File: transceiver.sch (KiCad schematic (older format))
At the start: 18 parts, among them U3 CC1200, Y1 Crystal_GND23

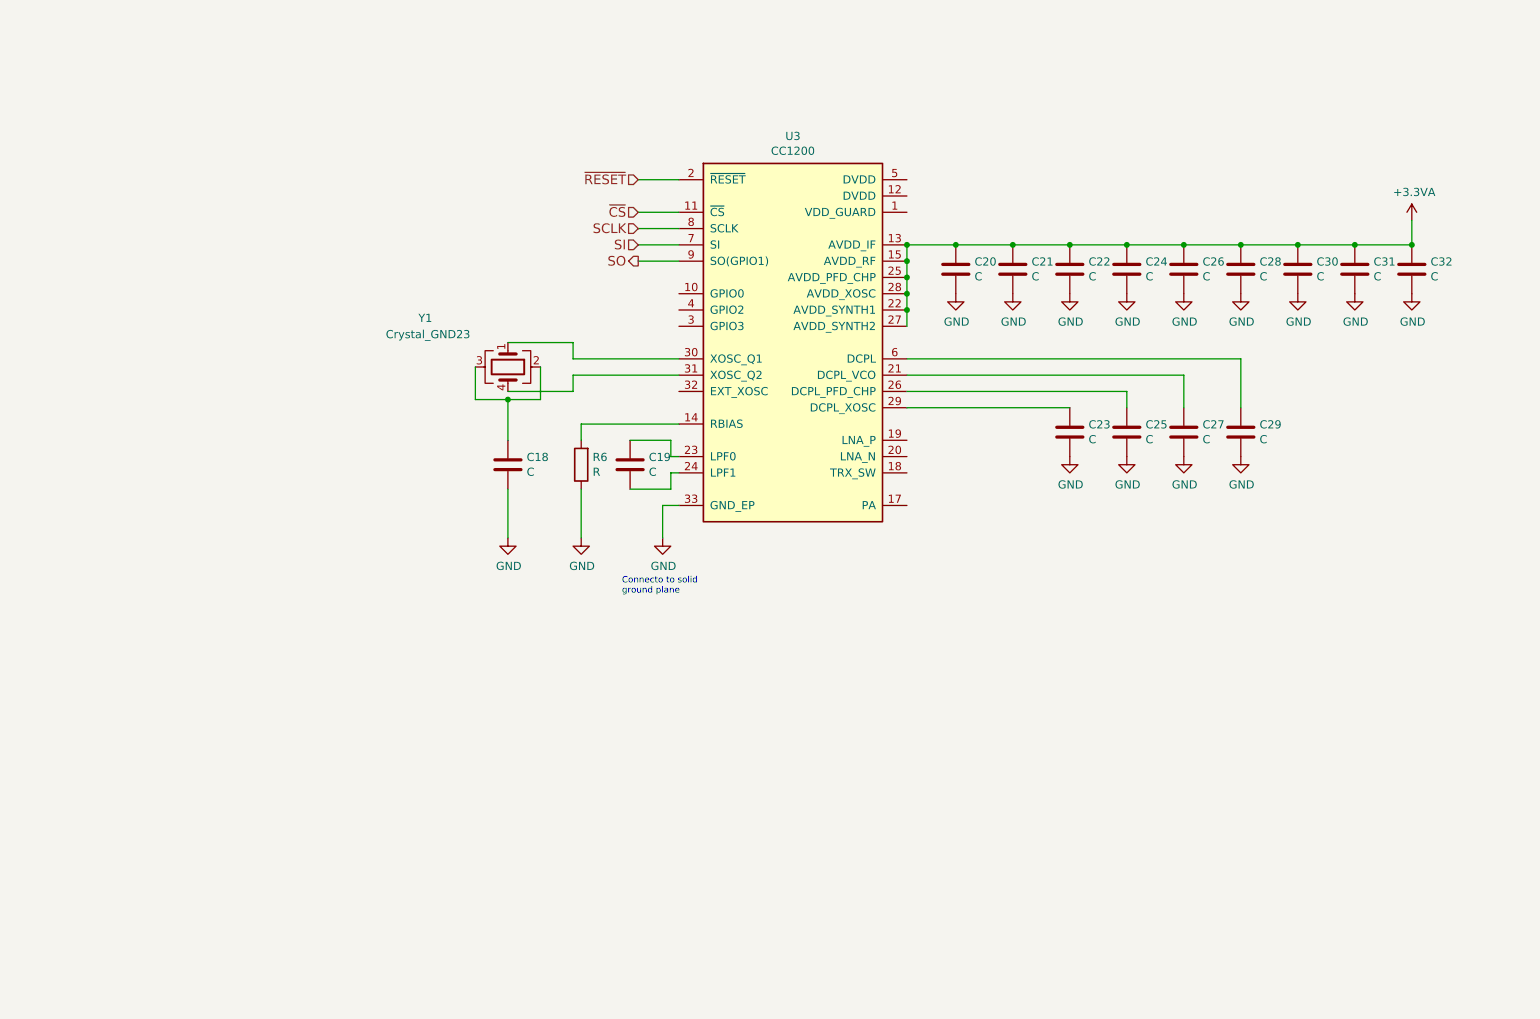
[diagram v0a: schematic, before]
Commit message: More work on tranciever and PA
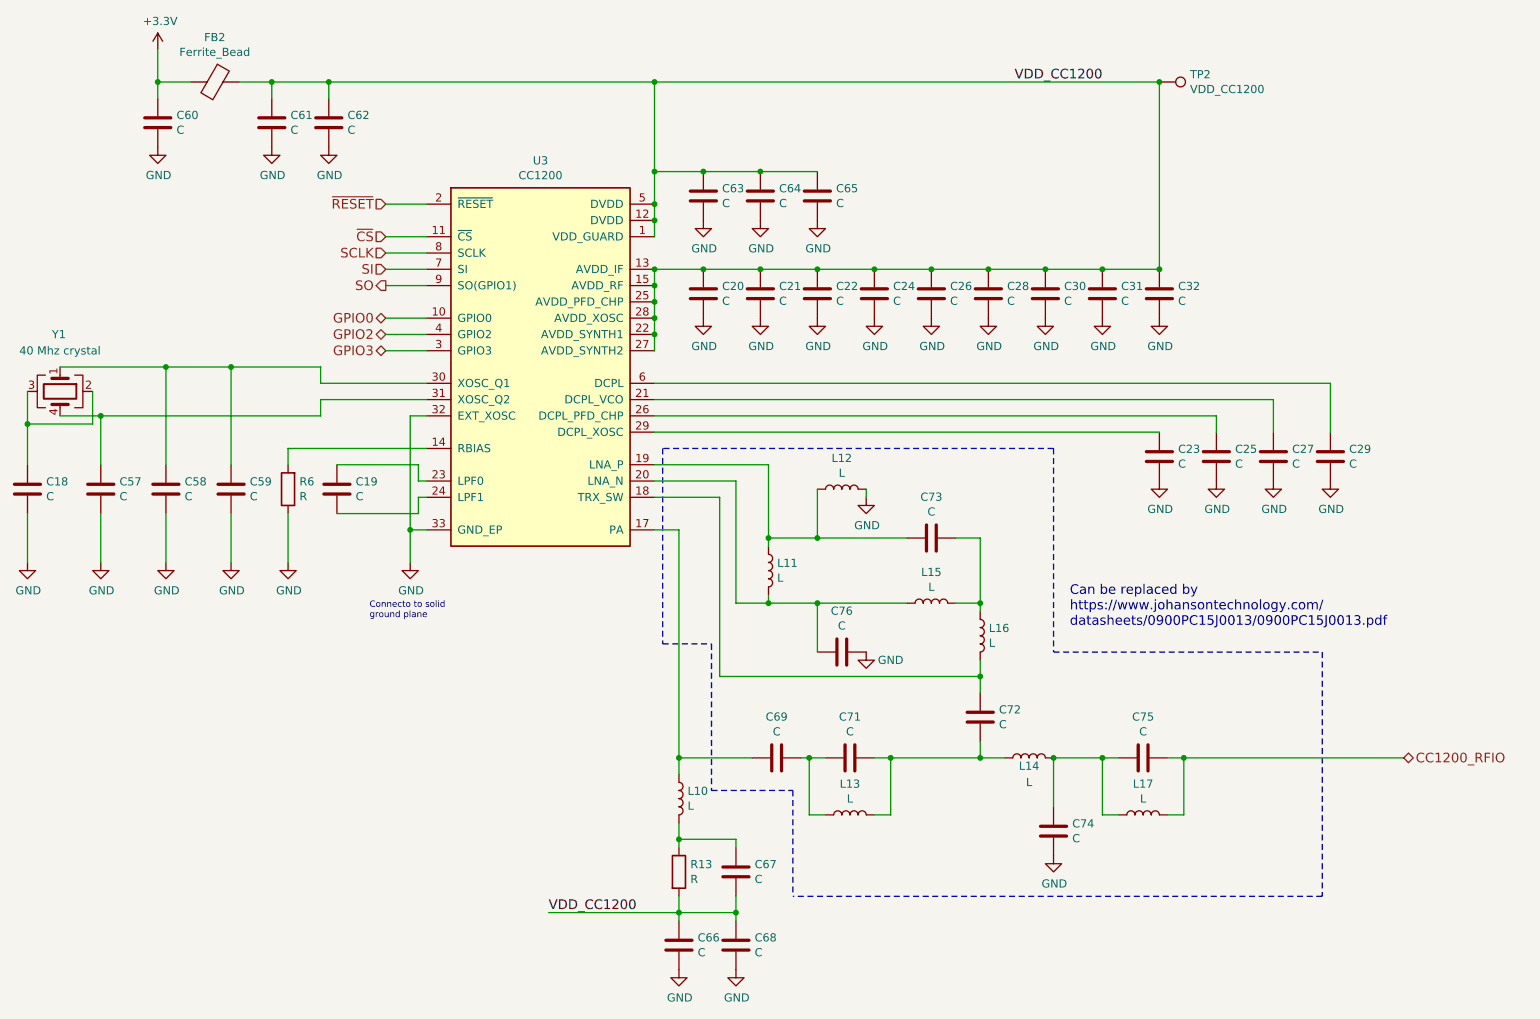
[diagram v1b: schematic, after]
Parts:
- added C57, C58, C59, C60, C61, C62, C63, C64, C65, C66, C67, C68, C69, C71, C72, C73, C74, C75, C76: C, symbol Device:C
- added FB2: Ferrite_Bead, symbol Device:Ferrite_Bead
- added L10, L11, L12, L13, L14, L15, L16, L17: L, symbol Device:L
- added R13: R, symbol Device:R
- added TP2: VDD_CC1200, symbol Connector:TestPoint
- Y1: value Crystal_GND23 -> 40 Mhz crystal
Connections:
- net +3.3VA is gone; now on net VDD_CC1200: C20.1, C21.1, C22.1, C24.1, C26.1, C28.1, C30.1, C31.1, C32.1, U3.13 (AVDD_IF), U3.15 (AVDD_RF), U3.22 (AVDD_SYNTH1), U3.25 (AVDD_PFD_CHP), U3.27 (AVDD_SYNTH2), U3.28 (AVDD_XOSC)
- net GND: now also U3.32 (EXT_XOSC), C57.2, C58.2, C59.2, C60.2, C61.2, C62.2, C63.2, C64.2, C65.2, C66.2, C68.2, C74.2, C76.1, L12.2
- net VDD_CC1200: now reaches U3.1 (VDD_GUARD)
- net VDD_CC1200: now also U3.12 (DVDD), U3.5 (DVDD), C61.1, C62.1, C63.1, C64.1, C65.1, C66.1, C67.2, C68.1, FB2.1, R13.2, TP2.1
- net GPIO0: now reaches U3.10 (GPIO0)
- net at U3.17 (PA): now also C69.2, L10.1
- net at U3.18 (TRX_SW): now also C72.1, L16.2
- net at U3.19 (LNA_P): now also C73.2, L11.1, L12.1
- net at U3.20 (LNA_N): now also C76.2, L11.2, L15.1
- net GPIO3: now reaches U3.3 (GPIO3)
- net at U3.30 (XOSC_Q1), Y1.1: now also C58.1, C59.1
- net at U3.31 (XOSC_Q2), Y1.4: now also C57.1
- net GPIO2: now reaches U3.4 (GPIO2)
- new net: C67.1, L10.2, R13.1
- new net: C69.1, C71.2, L13.1
- new net: C71.1, C72.2, L13.2, L14.1
- new net: C74.1, C75.2, L14.2, L17.1
- new net: C73.1, L15.2, L16.1
- new net +3V3: C60.1, FB2.2
- new net CC1200_RFIO: C75.1, L17.2
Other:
- note added: "Can be replaced by \nhttps://www.johansontechnology.com/\ndatasheets/0900PC15J0013/0900PC15J0013.pdf"
- moved on the sheet: C18, C19, C20, C21, C22, C23, C24, C25, C26, C27, C28, C29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
